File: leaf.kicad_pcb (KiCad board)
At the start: 6 copper layers, 49.8 x 49.7 mm, 292 parts, among them J1 Micro_SD_Card_Det1, J2 MIPI-CSI, J3 USB_OTG, Q1 Q_PNP_BEC, SW1 SKSGPAE010, SW2 SKSGPAE010, U1 BL8039, U2 rv1126/rv1109, U3 MTFC4GACAJCN, U4 AP6526, U5 RK809-2, U6 NCP114AMX250TCG, U7 Samsung K4A4G165WE-BCRC, U8 Samsung K4A4G165WE-BCRC, Y2 32.768kHz ±20ppm 12.5pF, Y3 24MHz ±10ppm 10pF

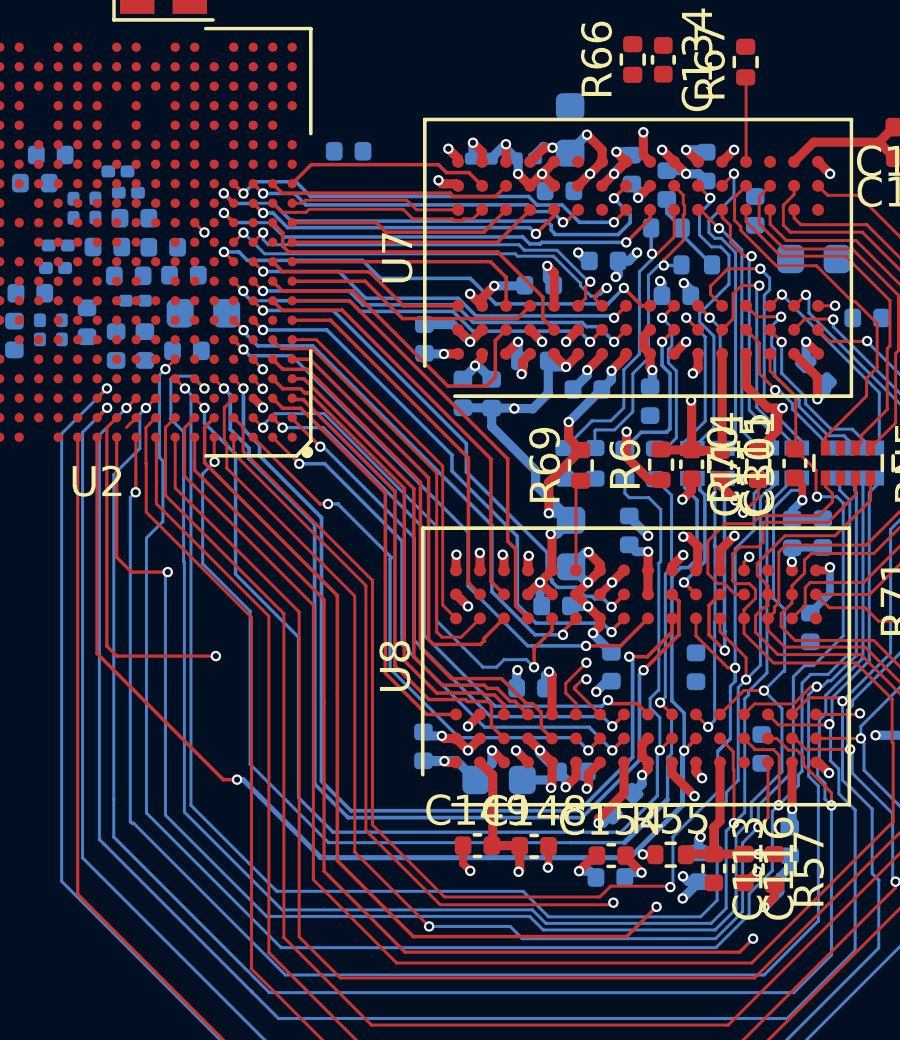
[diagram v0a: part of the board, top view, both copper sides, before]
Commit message: updated routes
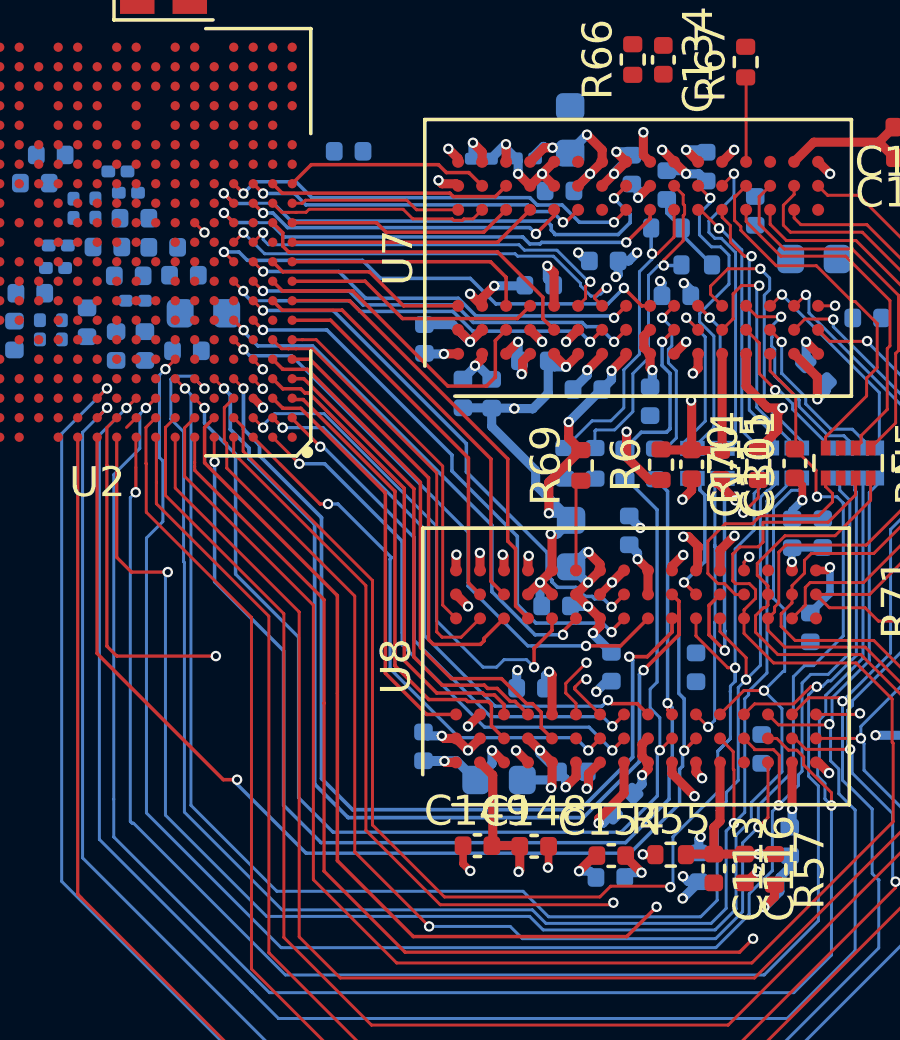
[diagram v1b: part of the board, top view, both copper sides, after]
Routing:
- net /DDR/DDR4_A14_~{WE}: track 42.6 -> 37.3 mm
- net /DDR/DDR4_ODT0: track 39.2 -> 38.7 mm
